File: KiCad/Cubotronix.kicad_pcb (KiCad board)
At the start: 2 copper layers, 35 x 35 mm, 32 parts, among them J1 Vin, J2 ADC, J3 GPIO12, J4 GPIO15, P2 Battery, P5 USB-Serial, P6 I2C/1-W, SW1 Boot, SW2 Reset, U1 AP2114H-3.3TRG1, U2 MCP73831T-2ATI/OT, U3 ESP-12E

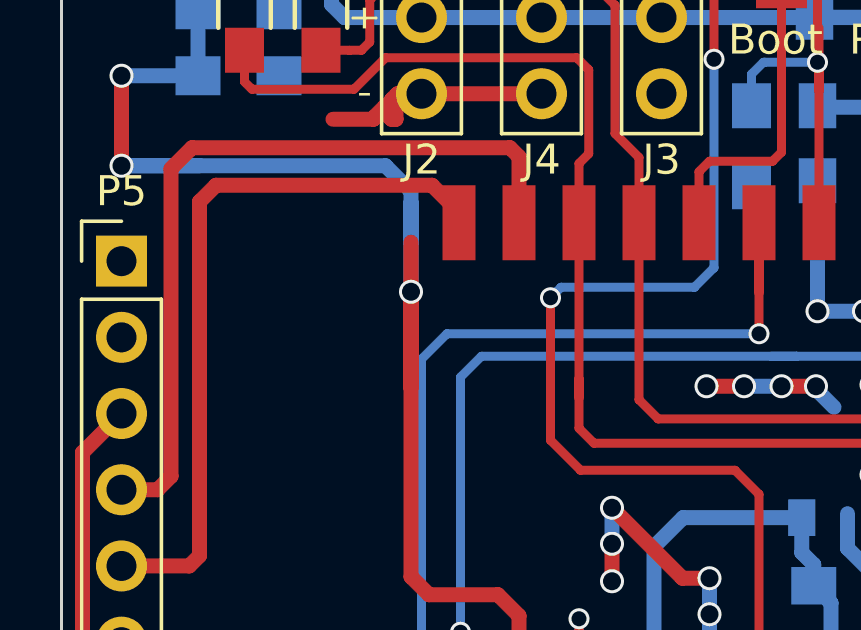
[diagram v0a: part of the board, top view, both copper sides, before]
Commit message: add gerber
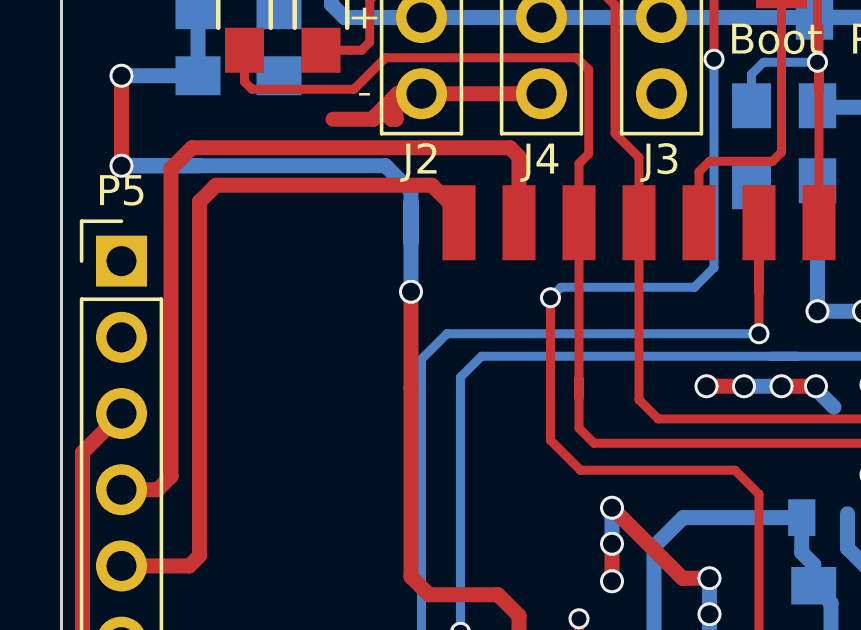
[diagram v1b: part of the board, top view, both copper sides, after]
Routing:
- net /ADC: track 46.1 -> 41.2 mm
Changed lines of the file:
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@@
   (general
     (links 66)
-    (no_connects 2)
-    (area 114.949999 54.949999 150.050001 90.050001)
+    (no_connects 1)
+    (area 82.150001 53.07619 150.125001 97.700001)
     (thickness 1.6)
     (drawings 30)
-    (tracks 363)
+    (tracks 362)
     (zones 0)
     (modules 32)
@@
   )
   (layers
-    (0 F.Cu signal hide)
-    (31 B.Cu signal hide)
-    (32 B.Adhes user)
-    (33 F.Adhes user)
-    (34 B.Paste user)
-    (35 F.Paste user)
+    (0 F.Cu signal)
+    (31 B.Cu signal)
+    (32 B.Adhes user hide)
+    (33 F.Adhes user hide)
+    (34 B.Paste user hide)
+    (35 F.Paste user hide)
     (36 B.SilkS user)
     (37 F.SilkS user)
     (38 B.Mask user)
     (39 F.Mask user)
-    (40 Dwgs.User user)
-    (41 Cmts.User user)
-    (42 Eco1.User user)
-    (43 Eco2.User user)
+    (40 Dwgs.User user hide)
+    (41 Cmts.User user hide)
+    (42 Eco1.User user hide)
+    (43 Eco2.User user hide)
     (44 Edge.Cuts user)
     (45 Margin user)
@@
     (47 F.CrtYd user)
     (48 B.Fab user hide)
-    (49 F.Fab user)
+    (49 F.Fab user hide)
   )
   (setup
@@
     (visible_elements FFFFFF7F)
     (pcbplotparams
-      (layerselection 0x010f0_80000001)
+      (layerselection 0x0d0f0_80000001)
       (usegerberextensions false)
       (excludeedgelayer true)
@@
       (drillshape 0)
       (scaleselection 1)
-      (outputdirectory "../Tarjetas Produccion/Gerbers_170109/LoRaKitty/"))
+      (outputdirectory "/Volumes/Macintosh_HD/Documents/Eduardo_ Contreras_Flores/Cubotronix/Gerbers/"))
   )
   (net 0 "")
@@
   (segment (start 125.3 84.95) (end 125.95 84.3) (width 0.3) (layer B.Cu) (net 17))
   (segment (start 126.65 67.95) (end 126.65 67) (width 0.5) (layer B.Cu) (net 18))
-  (segment (start 126.65 72.8) (end 126.65 67.95) (width 0.5) (layer F.Cu) (net 18))
   (via (at 126.65 69.6) (size 0.8) (drill 0.6) (layers F.Cu B.Cu) (net 18))
   (segment (start 126.65 69.6) (end 126.65 67) (width 0.5) (layer B.Cu) (net 18))
